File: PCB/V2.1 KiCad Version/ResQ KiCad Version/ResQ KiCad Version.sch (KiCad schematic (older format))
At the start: 8 parts, among them J1 Spare 1, J2 Spare 2, J3 OLED, J4 SD Card, J5 GPS, U1 WeMos_D1_mini

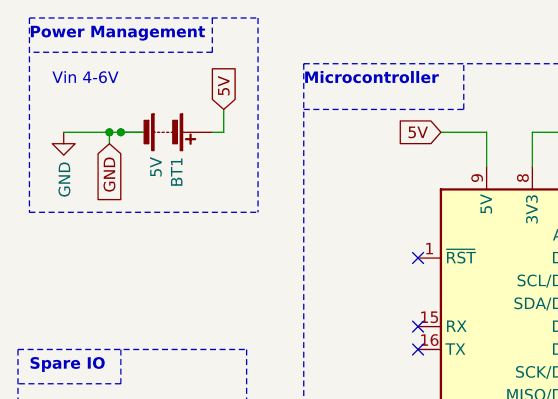
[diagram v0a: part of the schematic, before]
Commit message: v
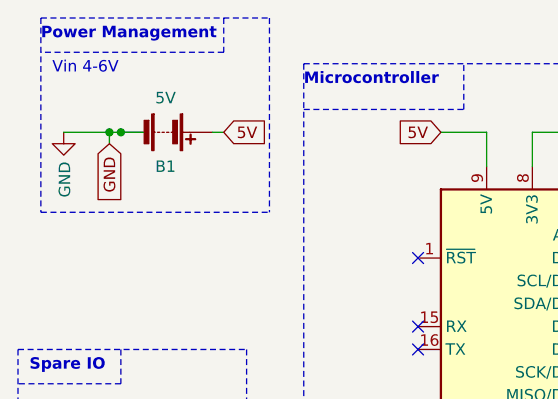
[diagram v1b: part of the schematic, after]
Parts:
- renumbered BT1 to B1
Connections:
- wire segments 23 -> 22
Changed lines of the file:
@@
 Sheet 1 1
 Title "ResQ Open Source Search and Rescue Hardware"
-Date "2020-08-10"
+Date "2020-08-17"
 Rev "2.1"
 Comp "MKME Lab"
@@
 	4850 4800 5850 4800
 Wire Notes Line
-	5700 3500 4900 3500
-Wire Notes Line
-	5700 3350 5700 3500
-Wire Notes Line
-	4900 3350 4900 4200
-Wire Notes Line
-	5900 3350 5900 4200
-Wire Notes Line
-	4900 3350 5900 3350
+	5750 3500 4950 3500
+Wire Notes Line
+	5750 3350 5750 3500
+Wire Notes Line
+	4950 3350 4950 4200
+Wire Notes Line
+	5950 3350 5950 4200
+Wire Notes Line
+	4950 3350 5950 3350
 Wire Notes Line
 	6100 3550 6100 5950
@@
 Wire Notes Line
 	8200 3350 8200 4450
-Text Notes 4900 3450 0    50   ~ 10
+Text Notes 4950 3450 0    50   ~ 10
 Power Management
 Text Notes 6100 3650 0    50   ~ 10
@@
 SDA
 Wire Notes Line
-	4900 4200 5900 4200
-Text Notes 5000 3650 0    50   ~ 0
+	4950 4200 5950 4200
+Text Notes 5000 3600 0    50   ~ 0
 Vin 4-6V
 Text GLabel 6700 3850 0    50   Input ~ 0
@@
 Text Notes 9450 4900 0    50   ~ 0
 Note:\n10K pullup not always needed \nbut without can cause random \nwrite errors
-Text GLabel 5750 3750 1    50   Input ~ 0
+Text GLabel 5750 3850 2    50   Input ~ 0
 5V
 Text GLabel 5250 3900 3    50   Input ~ 0
@@
 $EndComp
 $Comp
-L Device:Battery BT1
+L Device:Battery B1
 U 1 1 5F31A8A9
 P 5500 3850
-F 0 "BT1" H 5608 3896 50  0000 L CNN
-F 1 "5V" H 5608 3805 50  0000 L CNN
+F 0 "B1" V 5650 3800 50  0000 L CNN
+F 1 "5V" V 5350 3800 50  0000 L CNN
 F 2 "Connector_PinSocket_2.54mm:PinSocket_1x02_P2.54mm_Vertical" V 5500 3910 50  0001 C CNN
 F 3 "~" V 5500 3910 50  0001 C CNN
@@
 	5250 3850 5250 3900
 Wire Wire Line
-	5750 3750 5750 3850
-Wire Wire Line
 	5750 3850 5700 3850
